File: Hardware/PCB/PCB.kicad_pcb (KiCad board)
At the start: 4 copper layers, 72 parts, among them CN1 XT30UPB-M, J1 Connector, USB-TYPE-C-16P, SW1 TS-1187A-B-A-B, U1 RP2350B_C42415655, U10 KF128-2.54-3P, U11 KF128-2.54-3P, U12 KF128-2.54-3P, U2 KF128-2.54-2P, U3 BMP581, U4 ICM-45686, U5 BQ25883RGER, U6 LMR51430YFDDCR, U7 TPS630701RNMR, U8 GD25Q128ESIGR, U9 KF128-2.54-3P, X2 X322512MSB4SI

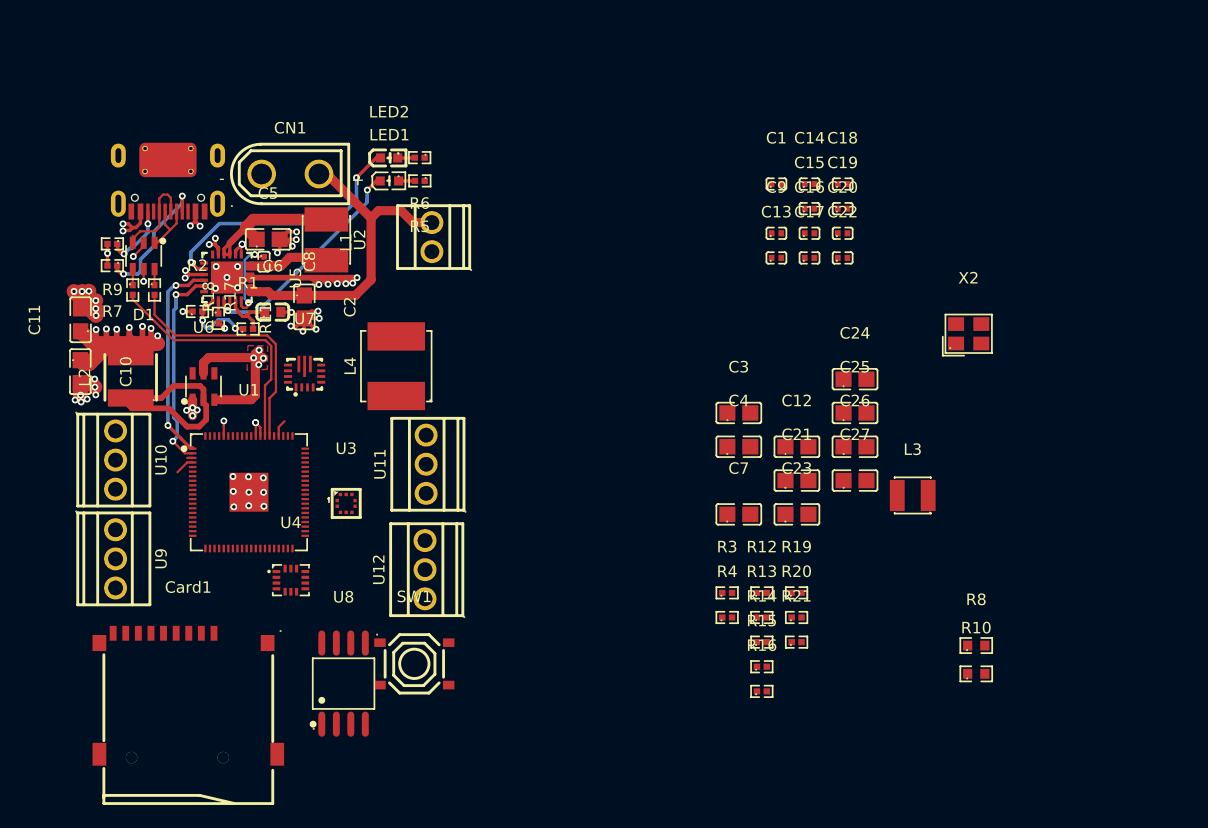
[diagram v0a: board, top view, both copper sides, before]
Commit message: Restarting PCB, finished Flash memory application
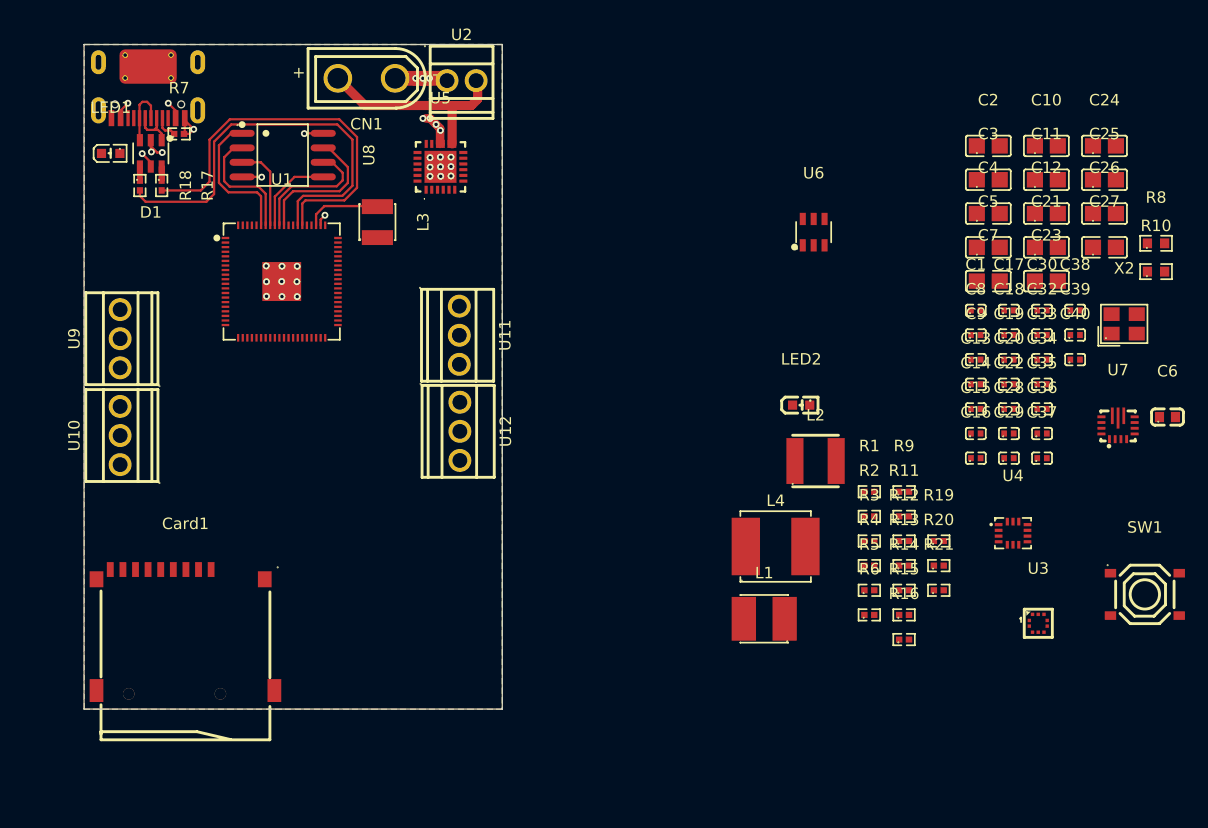
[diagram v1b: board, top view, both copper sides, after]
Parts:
- added C28: CL05B104KO5NNNC, easyeda2kicad:C0402, F.Cu at (105.8, 59.1)
- added C29: CL05B104KO5NNNC, easyeda2kicad:C0402, F.Cu at (105.8, 61.3)
- added C30: CL05B104KO5NNNC, easyeda2kicad:C0402, F.Cu at (108.7, 48.4)
- added C32: CL05B104KO5NNNC, easyeda2kicad:C0402, F.Cu at (108.7, 50.5)
- added C33: CL05B104KO5NNNC, easyeda2kicad:C0402, F.Cu at (108.7, 52.7)
- added C34: CL05B104KO5NNNC, easyeda2kicad:C0402, F.Cu at (108.7, 54.9)
- added C35: CL05B104KO5NNNC, easyeda2kicad:C0402, F.Cu at (108.7, 57.0)
- added C36: CL05B104KO5NNNC, easyeda2kicad:C0402, F.Cu at (108.7, 59.1)
- added C37: CL05B104KO5NNNC, easyeda2kicad:C0402, F.Cu at (108.7, 61.3)
- added C38: CL05B104KO5NNNC, easyeda2kicad:C0402, F.Cu at (111.6, 48.4)
- added C39: CL05B104KO5NNNC, easyeda2kicad:C0402, F.Cu at (111.6, 50.5)
- added C40: CL05B104KO5NNNC, easyeda2kicad:C0402, F.Cu at (111.6, 52.7)
- moved C10 86.6 mm to (109.1, 34.0), turned to 0 degrees
- moved C11 85.2 mm to (109.1, 37.0), turned to 0 degrees
- moved C6 78.6 mm to (119.7, 57.7)
- moved R9 72.4 mm to (96.7, 64.2), turned to 0 degrees
- moved U7 71.1 mm to (115.3, 58.6)
- moved SW1 64.0 mm to (117.7, 73.2)
- moved U4 63.2 mm to (106.2, 67.8)
- moved C5 62.8 mm to (104.0, 42.9)
- moved C8 62.5 mm to (102.9, 50.5), turned to 0 degrees
- moved R11 62.3 mm to (96.7, 66.4), turned to 0 degrees
- moved C2 61.3 mm to (104.0, 34.0), turned to 0 degrees
- moved U3 61.3 mm to (108.4, 75.7)
- moved R2 61.3 mm to (93.6, 66.4)
- moved L2 60.2 mm to (88.9, 61.5), turned to 0 degrees
- moved R1 56.0 mm to (93.6, 64.2)
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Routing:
- net +3V3: track 39.4 -> 1.66 mm, vias 10 -> 1
- net +7.5V: track 38.3 -> 3.46 mm, vias 10 -> 4
- net Net-(LED2-K): track 23.6 -> 0.00 mm, vias 2 -> 0
- net GND: track 36.3 -> 13.9 mm, vias 49 -> 26
- net Net-(LED1-K): track 19.6 -> 0.00 mm, vias 2 -> 0
- net Net-(U6-SW): track 19.0 -> 0.00 mm
- net Net-(U1-GPIO4): track 18.2 -> 0.00 mm, vias 2 -> 0
- net Net-(U1-GPIO5): track 18.1 -> 0.00 mm, vias 2 -> 0
- net Net-(U1-USB_DP): track 22.2 -> 36.7 mm
- net Net-(C5-Pad1): track 13.2 -> 0.00 mm
- net Net-(U1-QSPI_SD3): track 0.00 -> 12.6 mm
- net Net-(U1-USB_DM): track 21.6 -> 34.1 mm
- net Net-(U1-QSPI_SS): track 0.00 -> 12.4 mm
- net +5V: track 19.7 -> 7.82 mm, vias 7 -> 3
- net Net-(U1-QSPI_SCLK): track 0.00 -> 11.2 mm
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- added copper zone on B.Cu, net GND
- added copper zone on F.Cu, net GND
- removed copper zone on In2.Cu, net (none)
- removed copper zone on In2.Cu, net +3V3
- removed copper zone on F.Cu, net +7.5V
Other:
- board outline added: 36.5 x 58 mm
